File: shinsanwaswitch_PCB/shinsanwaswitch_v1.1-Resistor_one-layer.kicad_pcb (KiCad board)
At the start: 2 copper layers, 26.3 x 15.4 mm, 9 parts, among them J1 Conn_01x05_Male, Q1 2SC5395

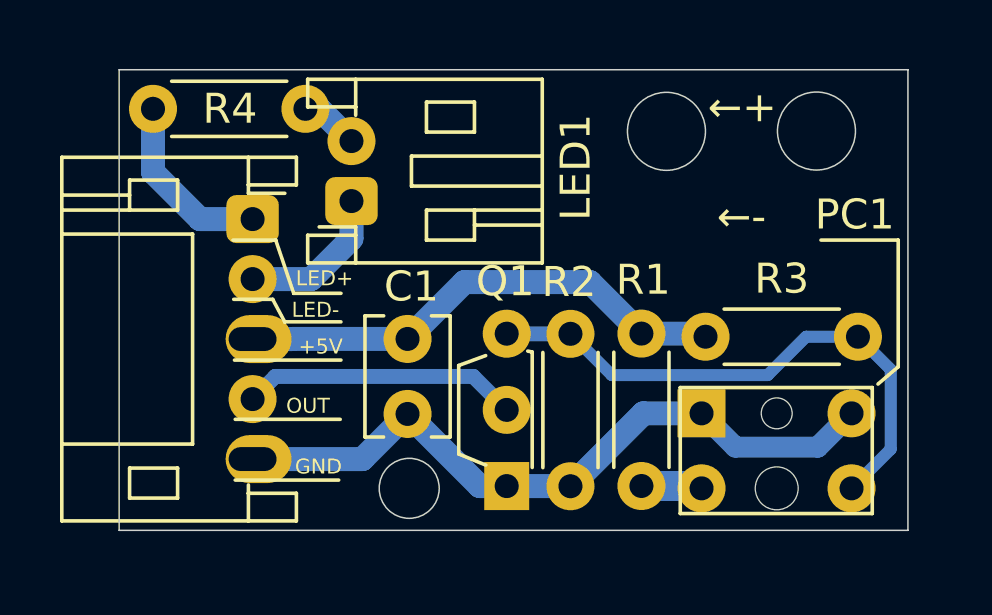
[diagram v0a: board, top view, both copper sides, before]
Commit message: Update for DIY-make boards
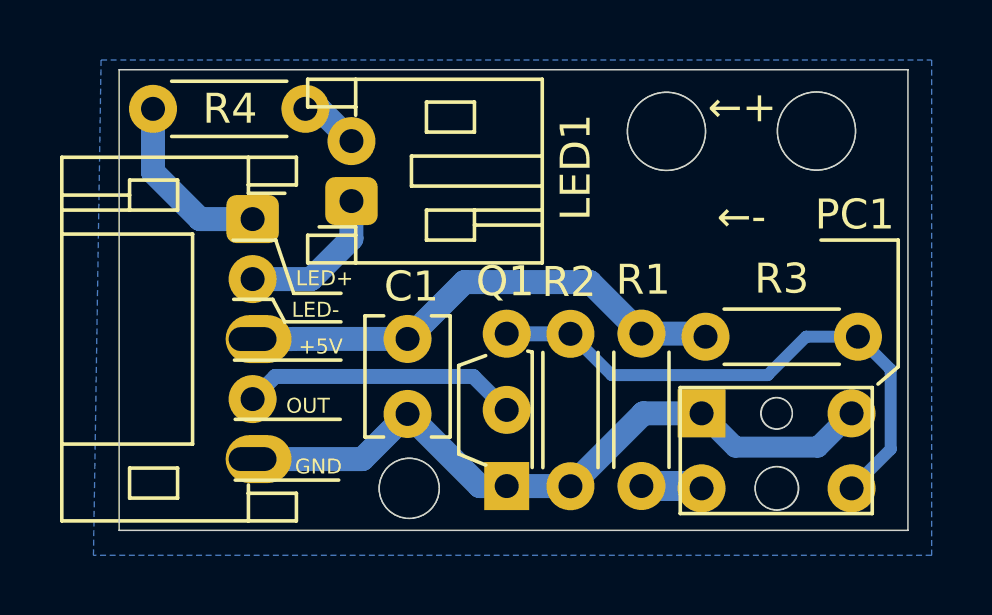
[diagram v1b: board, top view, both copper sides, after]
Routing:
- net (no net): vias 0 -> 5
- added copper zone on B.Cu, net (none)
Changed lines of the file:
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@@
     (effects (font (size 0.5 0.5) (thickness 0.125)))
   )
+  (via (at 146.1 76.8) (size 2.65) (drill 2.58) (layers "F.Cu" "B.Cu") (free) (net 0))
+  (via (at 149.77 86.2) (size 1.1) (drill 1) (layers "F.Cu" "B.Cu") (free) (net 0))
+  (via (at 137.525 88.7) (size 2.05) (drill 1.98) (layers "F.Cu" "B.Cu") (free) (net 0))
+  (via (at 149.78 88.7) (size 1.5) (drill 1.4) (layers "F.Cu" "B.Cu") (free) (net 0))
+  (via (at 151.1 76.79) (size 2.65) (drill 2.58) (layers "F.Cu" "B.Cu") (free) (net 0))
   (segment (start 151.145 87.325) (end 148.395 87.325) (width 0.7) (layer "B.Cu") (net 1))
   (segment (start 148.395 87.325) (end 147.27 86.2) (width 0.7) (layer "B.Cu") (net 1))
@@
   (segment (start 145.265299 83.541846) (end 147.298694 83.541846) (width 0.8) (layer "B.Cu") (net 8))
   (segment (start 137.47 83.72) (end 133.62 83.72) (width 0.8) (layer "B.Cu") (net 8))
+  (zone (net 0) (net_name "") (layer "B.Cu") (hatch edge 0.508)
+    (connect_pads (clearance 0.508))
+    (min_thickness 0.254) (filled_areas_thickness no)
+    (fill yes (thermal_gap 0.508) (thermal_bridge_width 0.508))
+    (polygon
+      (pts
+        (xy 154.94 90.932)
+        (xy 127 90.932)
+        (xy 127.254 74.422)
+        (xy 154.94 74.422)
+      )
+    )
+  )
 )
